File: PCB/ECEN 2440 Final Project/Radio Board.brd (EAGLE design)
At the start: 41.6 x 57.1 mm, 14 parts

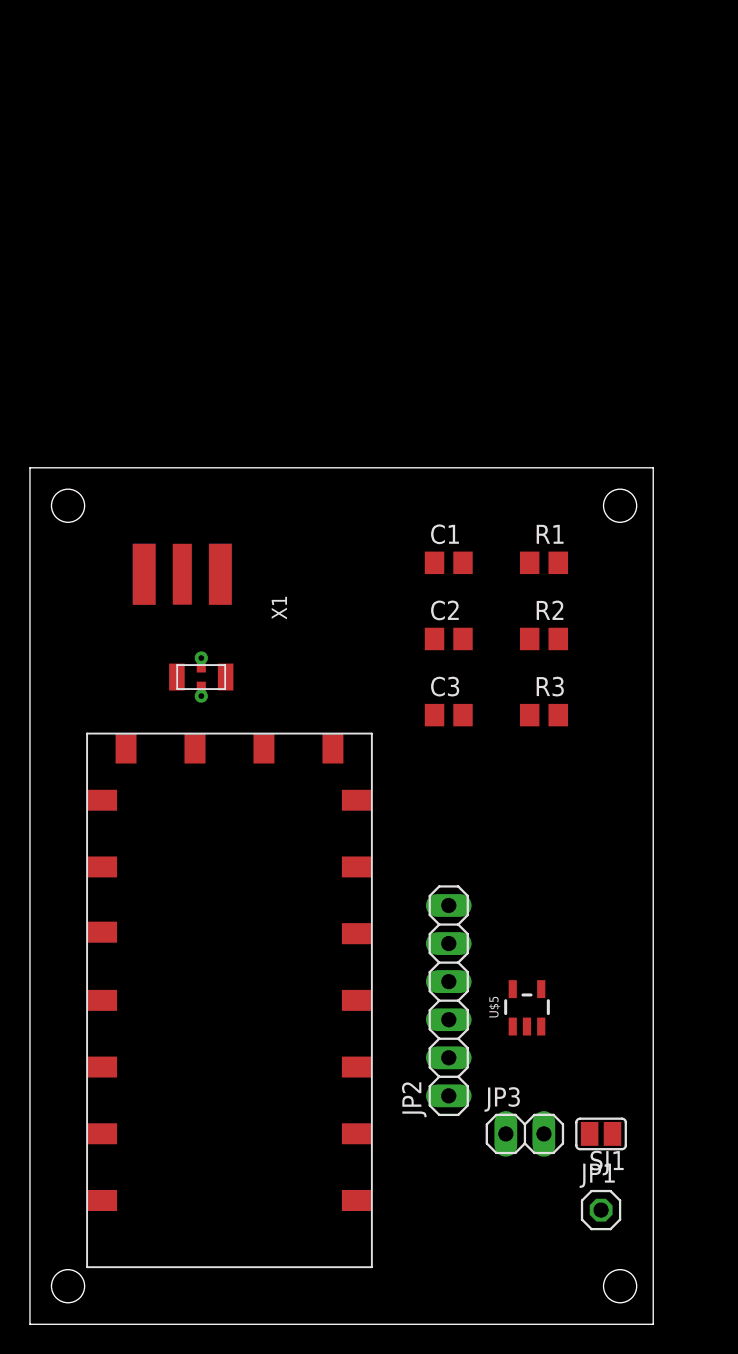
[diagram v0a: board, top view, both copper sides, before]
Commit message: Final updates to the board
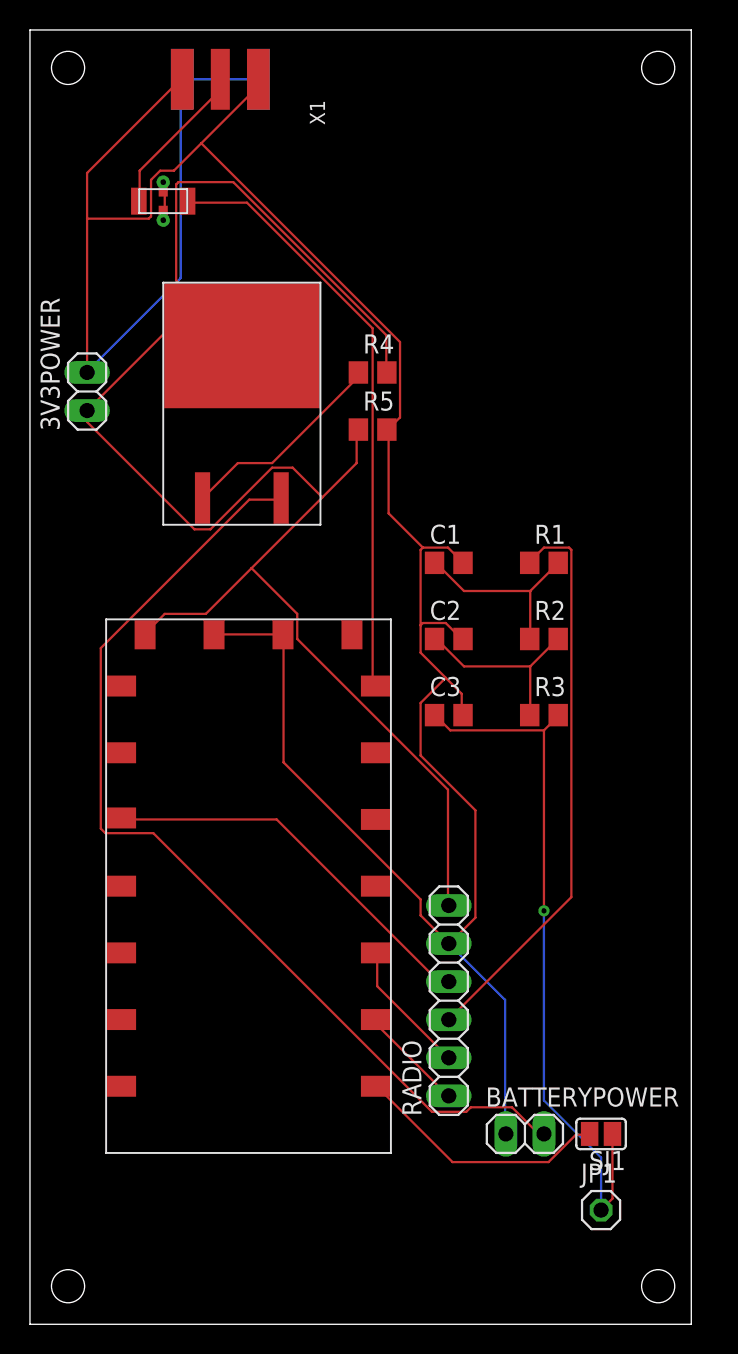
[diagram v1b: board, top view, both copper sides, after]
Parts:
- removed U$5: LDO-S-816, Custom Library:LDO-S-816
- added 3V3POWER: (no value), pinhead:1X02
- added LM317: LM317, Custom Library:LM317
- added R4, R5: 100R, rcl:R0805
- moved X1 33.1 mm to (12.7, 85.1)
- moved U$6 31.9 mm to (8.89, 74.9)
- moved U$4 7.73 mm to (5.08, 11.4)
- renumbered JP2 to RADIO, JP3 to BATTERYPOWER
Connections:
- new net N$8: LM317.ADJUST1, R4.1
- net +3V3: now also 3V3POWER.1, LM317.VOUT, R4.2, R5.1
- net GND: now also 3V3POWER.2, R5.2; no longer U$5.VSS
- net VCC: now also LM317.VIN; no longer U$5.VIN
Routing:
- net GND: track 0.00 -> 184.1 mm
- net +3V3: track 0.00 -> 119.0 mm
- net VCC: track 0.00 -> 66.5 mm
- net N$3: track 0.00 -> 48.1 mm, vias 0 -> 1
- net N$1: track 0.00 -> 39.9 mm
- net AUDIO_PWM: track 0.00 -> 38.0 mm
- net AUDIO_PTT: track 0.00 -> 26.4 mm
- net N$5: track 0.00 -> 17.2 mm
- net N$8: track 0.00 -> 14.1 mm
- net N$2: track 0.00 -> 13.0 mm
- net N$4: track 0.00 -> 13.0 mm
- net N$6: track 0.00 -> 10.4 mm
- net RX_RADIO: track 0.00 -> 9.01 mm
- net TX_RADIO: track 0.00 -> 7.14 mm
- net GND1: track 0.00 -> 3.19 mm
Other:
- board size 41.6 x 57.1 mm -> 44.1 x 86.3 mm
